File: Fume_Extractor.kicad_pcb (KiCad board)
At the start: 2 copper layers, 40 x 60 mm, 25 parts, among them J1 USB_B_Micro, J2 Conn_01x02, J3 Conn_01x02, U1 SP34063AEN, U2 TP4056

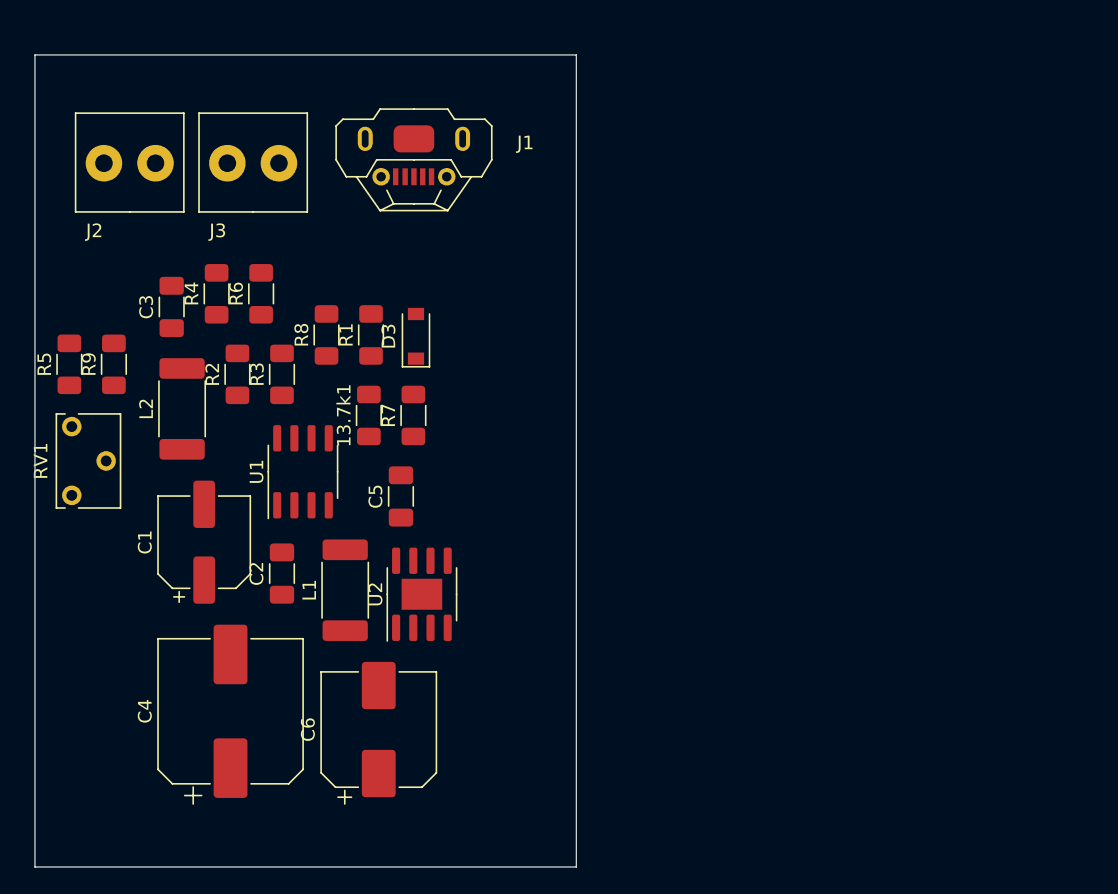
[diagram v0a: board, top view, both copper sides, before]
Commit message: Major schematic and layout updates
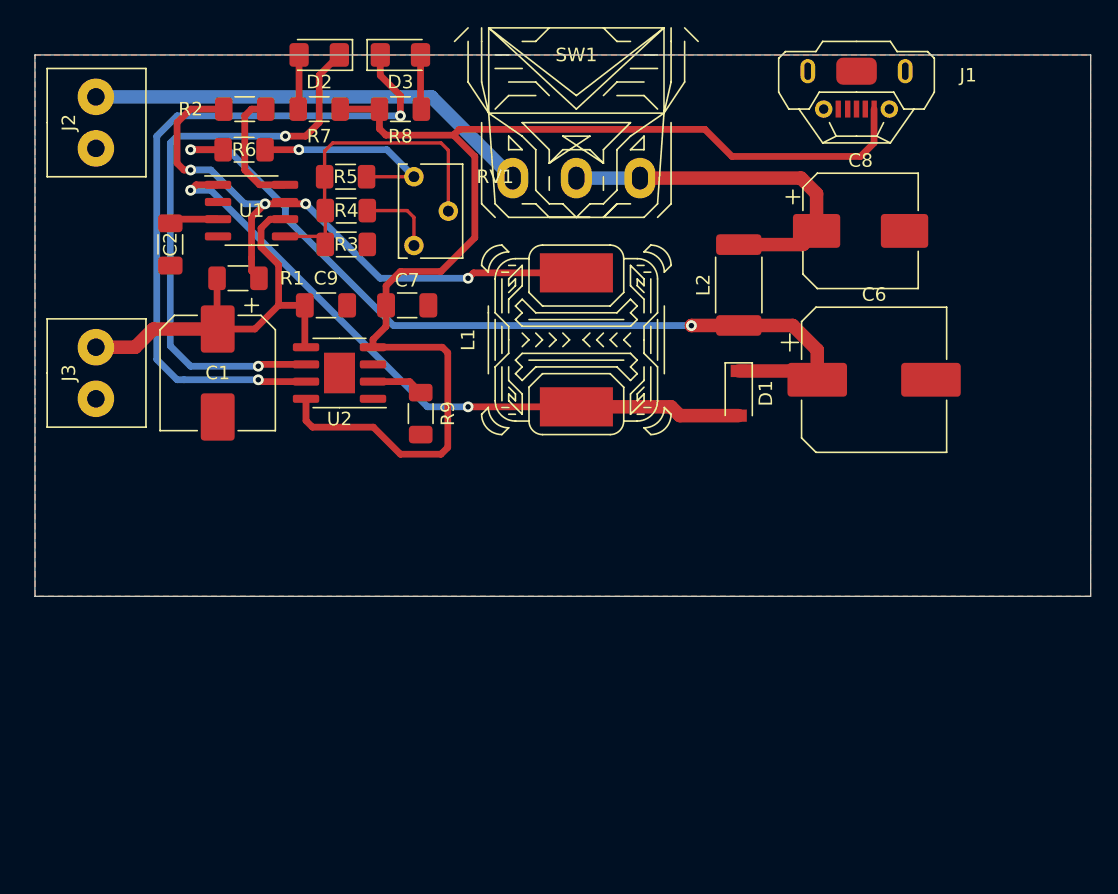
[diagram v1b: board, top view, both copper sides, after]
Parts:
- removed 13.7k1: R2, Resistor_SMD:R_1206_3216Metric_Pad1.30x1.75mm_HandSolder
- removed C3: 1.5nF ±10% 50V X7R 1206, Capacitor_SMD:C_1206_3216Metric_Pad1.33x1.80mm_HandSolder
- removed C4: 330uF ±20% 50V, Capacitor_SMD:CP_Elec_10x12.5
- removed C5: 10uF, Capacitor_SMD:C_1206_3216Metric_Pad1.33x1.80mm_HandSolder
- added C7: 10uF, Capacitor_SMD:C_1206_3216Metric_Pad1.33x1.80mm_HandSolder, F.Cu at (27.5, 18.5)
- added C8: 100uF ±20% 50V, Capacitor_SMD:CP_Elec_8x10, F.Cu at (61.0, 13.0)
- added C9: 10uF, Capacitor_SMD:C_1206_3216Metric_Pad1.33x1.80mm_HandSolder, F.Cu at (21.5, 18.5)
- added D1: 40V 1A 450mV @ 1A, Diode_SMD:D_SOD-123, F.Cu at (52.0, 25.0)
- added D2: LED, Diode_SMD:D_1206_3216Metric_Pad1.42x1.75mm_HandSolder, F.Cu at (21.0, 0.00)
- added SW1: SW_SPDT, Fume_Extractor:Switch_SS-12D06L5, F.Cu at (40.0, -2.00)
- C1: value 100µF -> 100uF ±20% 50V; footprint Capacitor_SMD:CP_Elec_6.3x5.3 -> Capacitor_SMD:CP_Elec_8x10
- C2: value 10uF -> 1.5nF ±10% 50V X7R 1206
- C6: value 100uF ±20% 50V -> 330uF ±20% 50V; footprint Capacitor_SMD:CP_Elec_8x10 -> Capacitor_SMD:CP_Elec_10x12.5
- D3: value 40V 1A 450mV @ 1A -> LED; footprint Diode_SMD:D_SOD-123 -> Diode_SMD:D_1206_3216Metric_Pad1.42x1.75mm_HandSolder
- L1: value 150uH ±10% 6*8 Radial Inductor -> 150uH ±20% 1.42A 280mΩ; footprint Inductor_SMD:L_2512_6332Metric_Pad1.52x3.35mm_HandSolder -> Fume_Extractor:Inductor_SLH_12x12x8
- R1: value R1 -> 0.22 R
- R2: value 0.22 R -> 180R
- R3: value 10k -> 16k
- R4: value 180R -> 0R
- R5: value 48k -> 508.064k
- R6: value 10k -> 48k
- R7: value 118k -> 10k
- R8: value RProg -> 10k
- R9: value 508.064k -> 1.2 k
- RV1: value 500M -> 500k
- moved C6 44.8 mm to (62.0, 24.0), turned to 0 degrees
- moved L2 42.1 mm to (52.0, 17.0)
- moved J1 33.1 mm to (60.7, 4.00)
- moved RV1 31.3 mm to (28.0, 9.00)
- moved C2 25.7 mm to (10.0, 14.0), turned to 270 degrees
- moved L1 25.2 mm to (40.0, 21.1), turned to 180 degrees
- moved R5 24.7 mm to (22.9, 9.00), turned to 0 degrees
- moved R7 23.7 mm to (21.0, 4.00), turned to 0 degrees
- moved R9 23.0 mm to (28.5, 26.5)
- moved D3 20.8 mm to (27.0, 0.00), turned to 0 degrees
- moved U1 19.7 mm to (16.0, 11.5), turned to 0 degrees
- moved R2 19.6 mm to (15.5, 4.00), turned to 180 degrees
- moved J3 19.4 mm to (4.50, 23.5), turned to 270 degrees
- moved R8 17.6 mm to (27.0, 4.00), turned to 180 degrees
- moved U2 17.4 mm to (22.5, 23.5), turned to 180 degrees
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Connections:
- C1 pad 1: VCC -> VBATT
- C2 pad 1: +5V -> Net-(C2-Pad1)
- C6 pad 1: +12V -> Net-(C6-Pad1)
- D3 pad 1: Net-(C4-Pad1) -> Net-(D3-Pad1)
- J2 pad 1: VBATT -> Net-(J2-Pad1)
- J3 pad 1: +12V -> VBATT
- L1 pad 1: Net-(L1-Pad1) -> Net-(D1-Pad2)
- L1 pad 2: Net-(D3-Pad2) -> Net-(L1-Pad2)
- L2 pad 1: Net-(C4-Pad1) -> Net-(C6-Pad1)
- L2 pad 2: +12V -> +24V
- R1 pad 1: Net-(F2-Pad2) -> Net-(L1-Pad2)
- R1 pad 2: +5V -> VBATT
- R2 pad 1: Net-(L1-Pad1) -> Net-(R2-Pad1)
- R2 pad 2: VCC -> Net-(L1-Pad2)
- R3 pad 1: Net-(D1-Pad2) -> GND
- R3 pad 2: +5V -> Net-(R3-Pad2)
- R4 pad 2: Net-(L1-Pad1) -> Net-(R3-Pad2)
- R5 pad 1: Net-(R5-Pad1) -> Net-(R3-Pad2)
- R6 pad 1: Net-(D2-Pad2) -> Net-(R5-Pad2)
- R6 pad 2: +5V -> Net-(C6-Pad1)
- R7 pad 1: Net-(C4-Pad1) -> Net-(D2-Pad2)
- R7 pad 2: Net-(13.7k1-Pad2) -> +5V
- R8 pad 1: GND -> Net-(D3-Pad2)
- R8 pad 2: Net-(R8-Pad2) -> +5V
- R9 pad 1: Net-(R9-Pad1) -> GND
- R9 pad 2: Net-(R5-Pad1) -> Net-(R9-Pad2)
- RV1 pad 1: Net-(R5-Pad1) -> Net-(R5-Pad2)
- RV1 pad 2: Net-(R9-Pad1) -> Net-(R3-Pad2)
- RV1 pad 3: Net-(RV1-Pad3) -> Net-(R4-Pad1)
- U1 pad 1: Net-(D3-Pad2) -> Net-(D1-Pad2)
- U1 pad 3: Net-(C3-Pad1) -> Net-(C2-Pad1)
- U1 pad 5: Net-(13.7k1-Pad2) -> Net-(R3-Pad2)
- U1 pad 6: Net-(L1-Pad1) -> VBATT
- U1 pad 7: Net-(L1-Pad1) -> Net-(L1-Pad2)
- U1 pad 8: Net-(R4-Pad1) -> Net-(R2-Pad1)
- U2 pad 1: Net-(F2-Pad2) -> GND
- U2 pad 2: Net-(R8-Pad2) -> Net-(R9-Pad2)
- U2 pad 7: Net-(D2-Pad1) (its old number) -> Net-(D3-Pad1)
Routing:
- net +5V: track 0.00 -> 92.2 mm
- net Net-(C6-Pad1): track 0.00 -> 63.6 mm, vias 0 -> 2
- net Net-(D3-Pad1): track 0.00 -> 51.9 mm, vias 0 -> 2
- net Net-(D1-Pad2): track 0.00 -> 49.6 mm, vias 0 -> 2
- net Net-(L1-Pad2): track 0.00 -> 46.7 mm, vias 0 -> 4
- net Net-(D2-Pad1): track 0.00 -> 42.9 mm, vias 0 -> 2
- net Net-(J2-Pad1): track 0.00 -> 33.3 mm
- net VBATT: track 0.00 -> 31.9 mm
- net +24V: track 0.00 -> 27.1 mm
- net Net-(R3-Pad2): track 0.00 -> 24.3 mm
- net Net-(R5-Pad2): track 0.00 -> 15.3 mm, vias 0 -> 1
- net Net-(R2-Pad1): track 0.00 -> 9.19 mm
- net Net-(R4-Pad1): track 0.00 -> 5.74 mm
- net Net-(D3-Pad2): track 0.00 -> 4.03 mm
- net Net-(D2-Pad2): track 0.00 -> 4.03 mm
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- added copper zone on F.Cu, net GND
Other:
- board size 40 x 60 mm -> 78 x 40 mm
